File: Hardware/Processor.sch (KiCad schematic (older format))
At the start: 24 parts, among them J1 ICSP-CORTEX, J3 CONN-9, U6 STM32L100RBT6, X1 8MHz

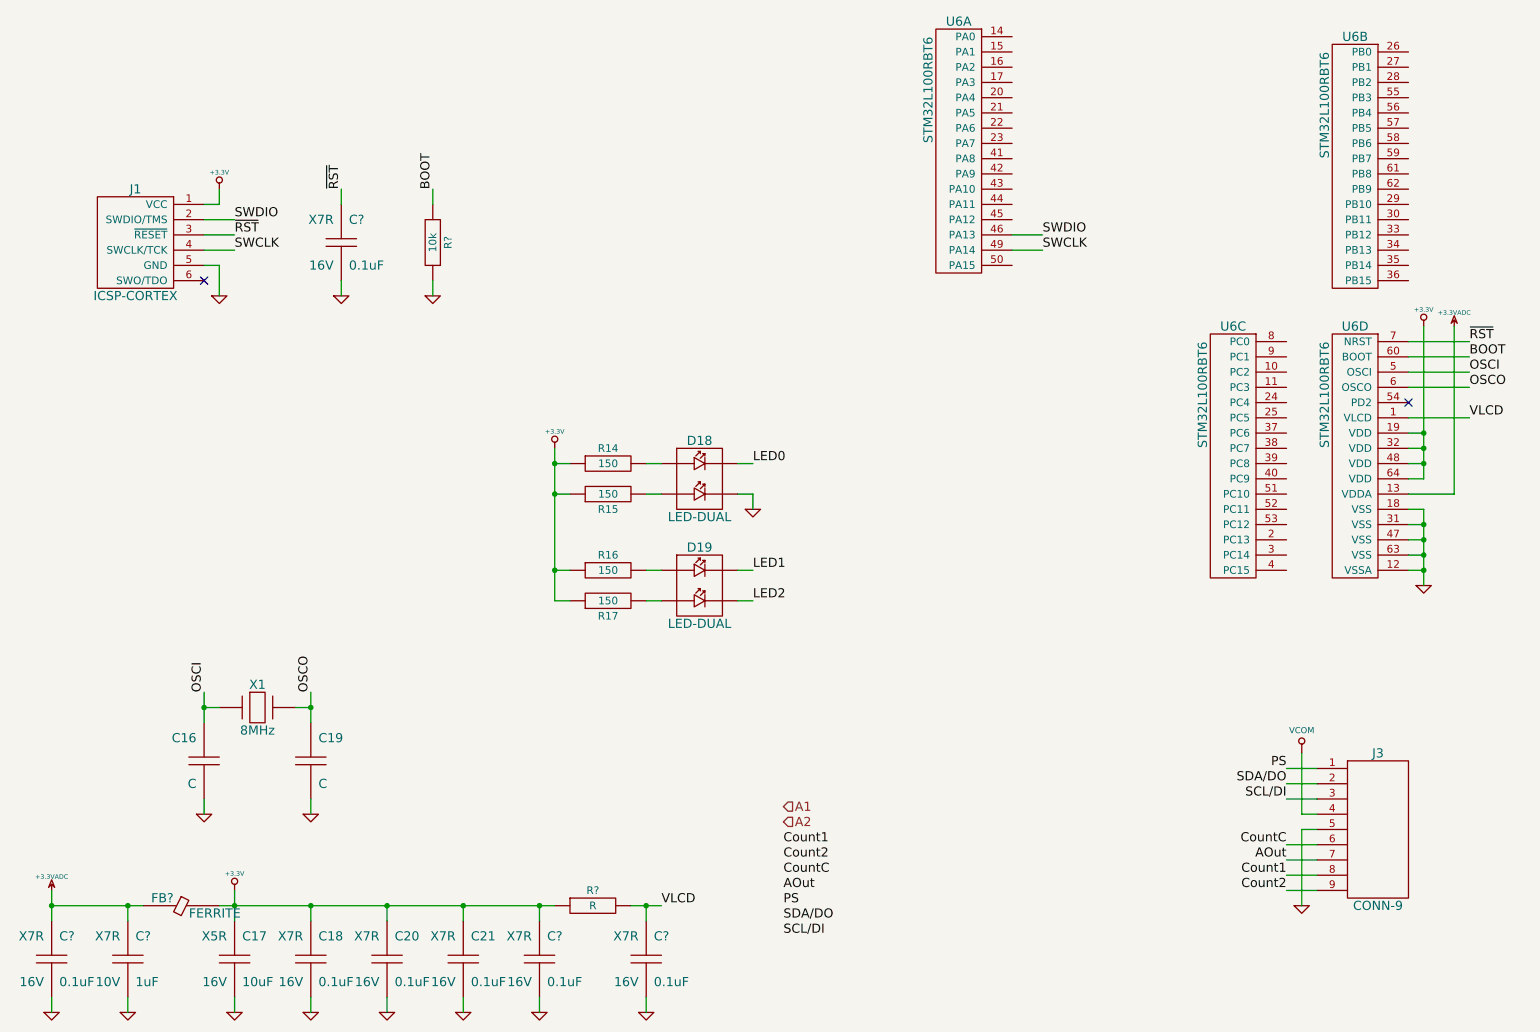
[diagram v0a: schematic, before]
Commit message: Component associations
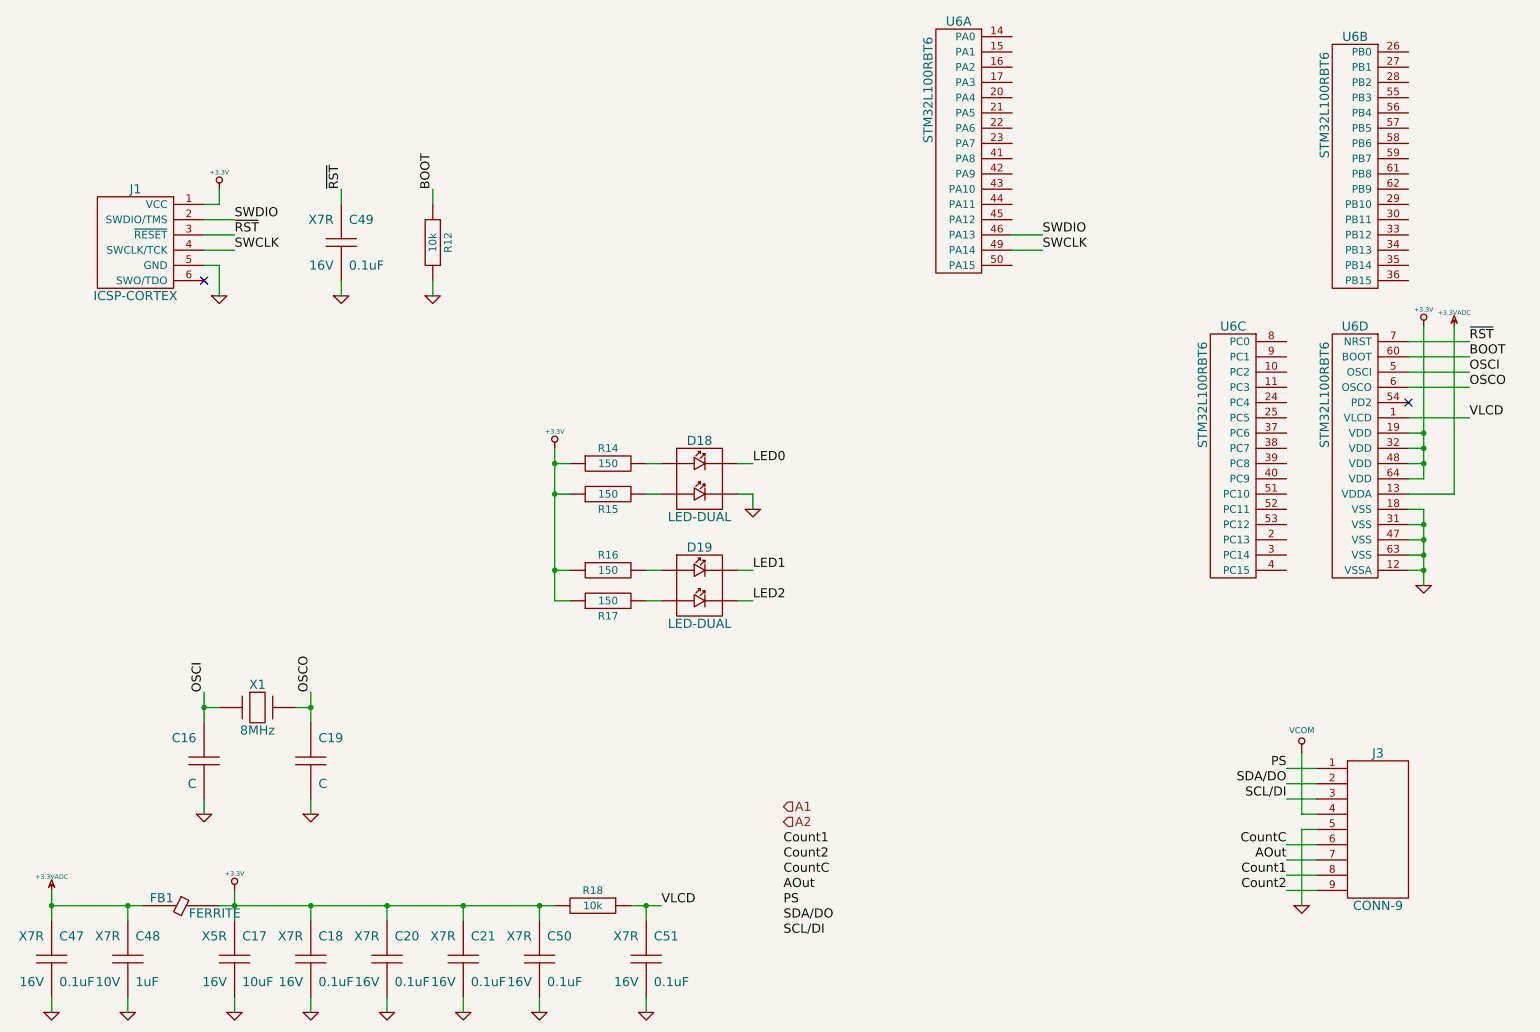
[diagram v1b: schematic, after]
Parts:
- removed R?: R, ~, symbol R
- added R18: 10k, RESC1608, symbol R
- gave numbers to parts that had none: 7
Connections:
- net +3.3V: now also R18.2
- net VLCD: now also R18.1
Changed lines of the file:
@@
 $EndComp
 $Comp
-L VCOM #PWR38
+L VCOM #PWR50
 U 1 1 52B50CC7
 P 9300 5500
-F 0 "#PWR38" H 9300 5700 40  0001 C CNN
+F 0 "#PWR50" H 9300 5700 40  0001 C CNN
 F 1 "VCOM" H 9300 5650 40  0000 C CNN
 F 2 "" H 9300 5500 60  0000 C CNN
@@
 LED0
 Wire Wire Line
-	2800 5100 2800 5200
-Wire Wire Line
-	2800 5200 2800 5300
-Wire Wire Line
-	2100 5100 2100 5200
-Wire Wire Line
-	2100 5200 2100 5300
+	2800 5100 2800 5300
+Wire Wire Line
+	2100 5100 2100 5300
 Wire Wire Line
 	2200 5200 2100 5200
@@
 	5700 3800 5600 3800
 Wire Wire Line
-	4400 3500 4400 3600
-Wire Wire Line
-	4400 3600 4400 3800
-Wire Wire Line
-	4400 3800 4400 4300
-Wire Wire Line
-	4400 4300 4400 4500
+	4400 3500 4400 4500
 Wire Wire Line
 	4400 4500 4500 4500
@@
 	2100 2200 2300 2200
 $Comp
-L C C?
+L C C50
 U 1 1 5411C9AD
 P 4300 6850
-F 0 "C?" H 4350 7000 60  0000 L CNN
+F 0 "C50" H 4350 7000 60  0000 L CNN
 F 1 "0.1uF" H 4350 6700 60  0000 L CNN
 F 2 "CAPC1608" H 4300 6850 60  0001 C CNN
@@
 $EndComp
 $Comp
-L C C?
+L C C48
 U 1 1 5411CA70
 P 1600 6850
-F 0 "C?" H 1650 7000 60  0000 L CNN
+F 0 "C48" H 1650 7000 60  0000 L CNN
 F 1 "1uF" H 1650 6700 60  0000 L CNN
 F 2 "CAPC1608" H 1600 6850 60  0001 C CNN
@@
 $EndComp
 $Comp
-L C C?
+L C C47
 U 1 1 5411CA9D
 P 1100 6850
-F 0 "C?" H 1150 7000 60  0000 L CNN
+F 0 "C47" H 1150 7000 60  0000 L CNN
 F 1 "0.1uF" H 1150 6700 60  0000 L CNN
 F 2 "CAPC1608" H 1100 6850 60  0001 C CNN
@@
 $EndComp
 $Comp
-L +3.3V #PWR?
+L +3.3V #PWR039
 U 1 1 5411CAA5
 P 2300 6400
-F 0 "#PWR?" H 2300 6360 30  0001 C CNN
+F 0 "#PWR039" H 2300 6360 30  0001 C CNN
 F 1 "+3.3V" H 2300 6510 30  0000 C CNN
 F 2 "" H 2300 6400 60  0000 C CNN
@@
 $EndComp
 Wire Wire Line
-	2300 6400 2300 6500
-Wire Wire Line
-	2300 6500 2300 6600
-$Comp
-L GND #PWR?
+	2300 6400 2300 6600
+$Comp
+L GND #PWR040
 U 1 1 5411CAE0
 P 2300 7200
-F 0 "#PWR?" H 2300 7200 30  0001 C CNN
+F 0 "#PWR040" H 2300 7200 30  0001 C CNN
 F 1 "GND" H 2300 7130 30  0001 C CNN
 F 2 "" H 2300 7200 60  0000 C CNN
@@
 $EndComp
 $Comp
-L GND #PWR?
+L GND #PWR041
 U 1 1 5411CAEF
 P 2800 7200
-F 0 "#PWR?" H 2800 7200 30  0001 C CNN
+F 0 "#PWR041" H 2800 7200 30  0001 C CNN
 F 1 "GND" H 2800 7130 30  0001 C CNN
 F 2 "" H 2800 7200 60  0000 C CNN
@@
 $EndComp
 $Comp
-L GND #PWR?
+L GND #PWR042
 U 1 1 5411CAFE
 P 3300 7200
-F 0 "#PWR?" H 3300 7200 30  0001 C CNN
+F 0 "#PWR042" H 3300 7200 30  0001 C CNN
 F 1 "GND" H 3300 7130 30  0001 C CNN
 F 2 "" H 3300 7200 60  0000 C CNN
@@
 $EndComp
 $Comp
-L GND #PWR?
+L GND #PWR043
 U 1 1 5411CB0D
 P 3800 7200
-F 0 "#PWR?" H 3800 7200 30  0001 C CNN
+F 0 "#PWR043" H 3800 7200 30  0001 C CNN
 F 1 "GND" H 3800 7130 30  0001 C CNN
 F 2 "" H 3800 7200 60  0000 C CNN
@@
 $EndComp
 $Comp
-L GND #PWR?
+L GND #PWR044
 U 1 1 5411CB1C
 P 4300 7200
-F 0 "#PWR?" H 4300 7200 30  0001 C CNN
+F 0 "#PWR044" H 4300 7200 30  0001 C CNN
 F 1 "GND" H 4300 7130 30  0001 C CNN
 F 2 "" H 4300 7200 60  0000 C CNN
@@
 $EndComp
 $Comp
-L GND #PWR?
+L GND #PWR045
 U 1 1 5411CB2B
 P 1600 7200
-F 0 "#PWR?" H 1600 7200 30  0001 C CNN
+F 0 "#PWR045" H 1600 7200 30  0001 C CNN
 F 1 "GND" H 1600 7130 30  0001 C CNN
 F 2 "" H 1600 7200 60  0000 C CNN
@@
 $EndComp
 $Comp
-L GND #PWR?
+L GND #PWR046
 U 1 1 5411CB3A
 P 1100 7200
-F 0 "#PWR?" H 1100 7200 30  0001 C CNN
+F 0 "#PWR046" H 1100 7200 30  0001 C CNN
 F 1 "GND" H 1100 7130 30  0001 C CNN
 F 2 "" H 1100 7200 60  0000 C CNN
@@
 $EndComp
 Wire Wire Line
-	1100 6400 1100 6500
-Wire Wire Line
-	1100 6500 1100 6600
+	1100 6400 1100 6600
 Connection ~ 2300 6500
 Wire Wire Line
@@
 	4300 7100 4300 7200
 $Comp
-L R R?
-U 1 1 5411CE1B
-P 4650 6500
-F 0 "R?" H 4650 6600 50  0000 C CNN
-F 1 "R" H 4650 6500 50  0000 C CNN
-F 2 "~" H 4650 6500 60  0000 C CNN
-F 3 "~" H 4650 6500 60  0000 C CNN
-F 4 "W" H 4650 6400 50  0001 C CNN "Power"
-F 5 "%" H 4650 6300 50  0001 C CNN "Tolerance"
-	1    4650 6500
-	1    0    0    -1
-$EndComp
-$Comp
-L C C?
+L C C51
 U 1 1 5411CE39
 P 5000 6850
-F 0 "C?" H 5050 7000 60  0000 L CNN
+F 0 "C51" H 5050 7000 60  0000 L CNN
 F 1 "0.1uF" H 5050 6700 60  0000 L CNN
 F 2 "CAPC1608" H 5000 6850 60  0001 C CNN
@@
 Connection ~ 4300 6500
 Wire Wire Line
-	4900 6500 5000 6500
-Wire Wire Line
-	5000 6500 5100 6500
+	4900 6500 5100 6500
 Wire Wire Line
 	5000 6500 5000 6600
 $Comp
-L GND #PWR?
+L GND #PWR047
 U 1 1 5411CEC2
 P 5000 7200
-F 0 "#PWR?" H 5000 7200 30  0001 C CNN
+F 0 "#PWR047" H 5000 7200 30  0001 C CNN
 F 1 "GND" H 5000 7130 30  0001 C CNN
 F 2 "" H 5000 7200 60  0000 C CNN
@@
 Connection ~ 5000 6500
 Wire Wire Line
-	1100 6500 1600 6500
-Wire Wire Line
-	1600 6500 1700 6500
-Wire Wire Line
-	2200 6500 2300 6500
-Wire Wire Line
-	2300 6500 2800 6500
-Wire Wire Line
-	2800 6500 3300 6500
-Wire Wire Line
-	3300 6500 3800 6500
-Wire Wire Line
-	3800 6500 4300 6500
-Wire Wire Line
-	4300 6500 4400 6500
-$Comp
-L FERRITE FB?
+	1100 6500 1700 6500
+Wire Wire Line
+	2200 6500 4400 6500
+$Comp
+L FERRITE FB1
 U 1 1 5411CFE1
 P 1950 6500
-F 0 "FB?" H 1900 6550 60  0000 R CNN
+F 0 "FB1" H 1900 6550 60  0000 R CNN
 F 1 "FERRITE" H 2000 6450 60  0000 L CNN
 F 2 "~" H 1950 6500 60  0000 C CNN
@@
 $EndComp
 $Comp
-L +3.3VADC #PWR?
+L +3.3VADC #PWR048
 U 1 1 5411D0AC
 P 1100 6400
-F 0 "#PWR?" H 1100 6520 20  0001 C CNN
+F 0 "#PWR048" H 1100 6520 20  0001 C CNN
 F 1 "+3.3VADC" H 1100 6490 30  0000 C CNN
 F 2 "" H 1100 6400 60  0000 C CNN
@@
 Connection ~ 1100 6500
 $Comp
-L +3.3VADC #PWR?
+L +3.3VADC #PWR049
 U 1 1 5411D101
 P 10300 2700
-F 0 "#PWR?" H 10300 2820 20  0001 C CNN
+F 0 "#PWR049" H 10300 2820 20  0001 C CNN
 F 1 "+3.3VADC" H 10300 2790 30  0000 C CNN
 F 2 "" H 10300 2700 60  0000 C CNN
@@
 $EndComp
 $Comp
-L +3.3V #PWR?
+L +3.3V #PWR050
 U 1 1 5411D110
 P 10100 2700
-F 0 "#PWR?" H 10100 2660 30  0001 C CNN
+F 0 "#PWR050" H 10100 2660 30  0001 C CNN
 F 1 "+3.3V" H 10100 2810 30  0000 C CNN
 F 2 "" H 10100 2700 60  0000 C CNN
@@
 $EndComp
 Wire Wire Line
-	10100 2700 10100 3400
-Wire Wire Line
-	10100 3400 10100 3500
-Wire Wire Line
-	10100 3500 10100 3600
-Wire Wire Line
-	10100 3600 10100 3700
+	10100 2700 10100 3700
 Wire Wire Line
 	10100 3400 10000 3400
@@
 	10400 3300 10000 3300
 $Comp
-L GND #PWR?
+L GND #PWR051
 U 1 1 5411D2E7
 P 10100 4400
-F 0 "#PWR?" H 10100 4400 30  0001 C CNN
+F 0 "#PWR051" H 10100 4400 30  0001 C CNN
 F 1 "GND" H 10100 4330 30  0001 C CNN
 F 2 "" H 10100 4400 60  0000 C CNN
@@
 $EndComp
 Wire Wire Line
-	10100 3900 10100 4000
-Wire Wire Line
-	10100 4000 10100 4100
-Wire Wire Line
-	10100 4100 10100 4200
-Wire Wire Line
-	10100 4200 10100 4300
-Wire Wire Line
-	10100 4300 10100 4400
+	10100 3900 10100 4400
 Wire Wire Line
 	10100 3900 10000 3900
@@
 NoConn ~ 10000 3200
 $Comp
-L C C?
+L C C49
 U 1 1 5411D10E
 P 3000 2150
-F 0 "C?" H 3050 2300 60  0000 L CNN
+F 0 "C49" H 3050 2300 60  0000 L CNN
 F 1 "0.1uF" H 3050 2000 60  0000 L CNN
 F 2 "CAPC1608" H 3000 2150 60  0001 C CNN
@@
 ~RST
 $Comp
-L GND #PWR?
+L GND #PWR052
 U 1 1 5411D116
 P 3000 2500
-F 0 "#PWR?" H 3000 2500 30  0001 C CNN
+F 0 "#PWR052" H 3000 2500 30  0001 C CNN
 F 1 "GND" H 3000 2430 30  0001 C CNN
 F 2 "" H 3000 2500 60  0000 C CNN
@@
 	3000 1900 3000 1800
 $Comp
-L R R?
+L R R12
 U 1 1 5411D395
 P 3600 2150
-F 0 "R?" H 3600 2250 50  0000 C CNN
+F 0 "R12" H 3600 2250 50  0000 C CNN
 F 1 "10k" H 3600 2150 50  0000 C CNN
 F 2 "RESC1608" H 3600 2150 60  0001 C CNN
@@
 $EndComp
 $Comp
-L GND #PWR?
+L GND #PWR053
 U 1 1 5411D3B1
 P 3600 2500
-F 0 "#PWR?" H 3600 2500 30  0001 C CNN
+F 0 "#PWR053" H 3600 2500 30  0001 C CNN
 F 1 "GND" H 3600 2430 30  0001 C CNN
 F 2 "" H 3600 2500 60  0000 C CNN
@@
 Wire Wire Line
 	7400 2200 7600 2200
+$Comp
+L R R18
+U 1 1 5411D7D0
+P 4650 6500
+F 0 "R18" H 4650 6600 50  0000 C CNN
+F 1 "10k" H 4650 6500 50  0000 C CNN
+F 2 "RESC1608" H 4650 6500 60  0001 C CNN
+F 3 "~" H 4650 6500 60  0000 C CNN
+F 4 "Yageo" H 4650 6500 60  0001 C CNN "MFR Name"
+F 5 "RC0603FR-0710KL" H 4650 6500 60  0001 C CNN "MFR Part No"
+F 6 "311-10.0KHRCT-ND" H 4650 6500 60  0001 C CNN "Distributor Part No"
+F 7 "0.1W" H 4650 6400 50  0001 C CNN "Power"
+F 8 "1%" H 4650 6300 50  0001 C CNN "Tolerance"
+	1    4650 6500
+	-1   0    0    -1
+$EndComp
 $EndSCHEMATC
